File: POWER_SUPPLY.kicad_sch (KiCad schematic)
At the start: 4 parts, among them J1 Jack-DC, J2 USB_B_Micro, U4 LMR33640ADDA, U5 LMR33640ADDA

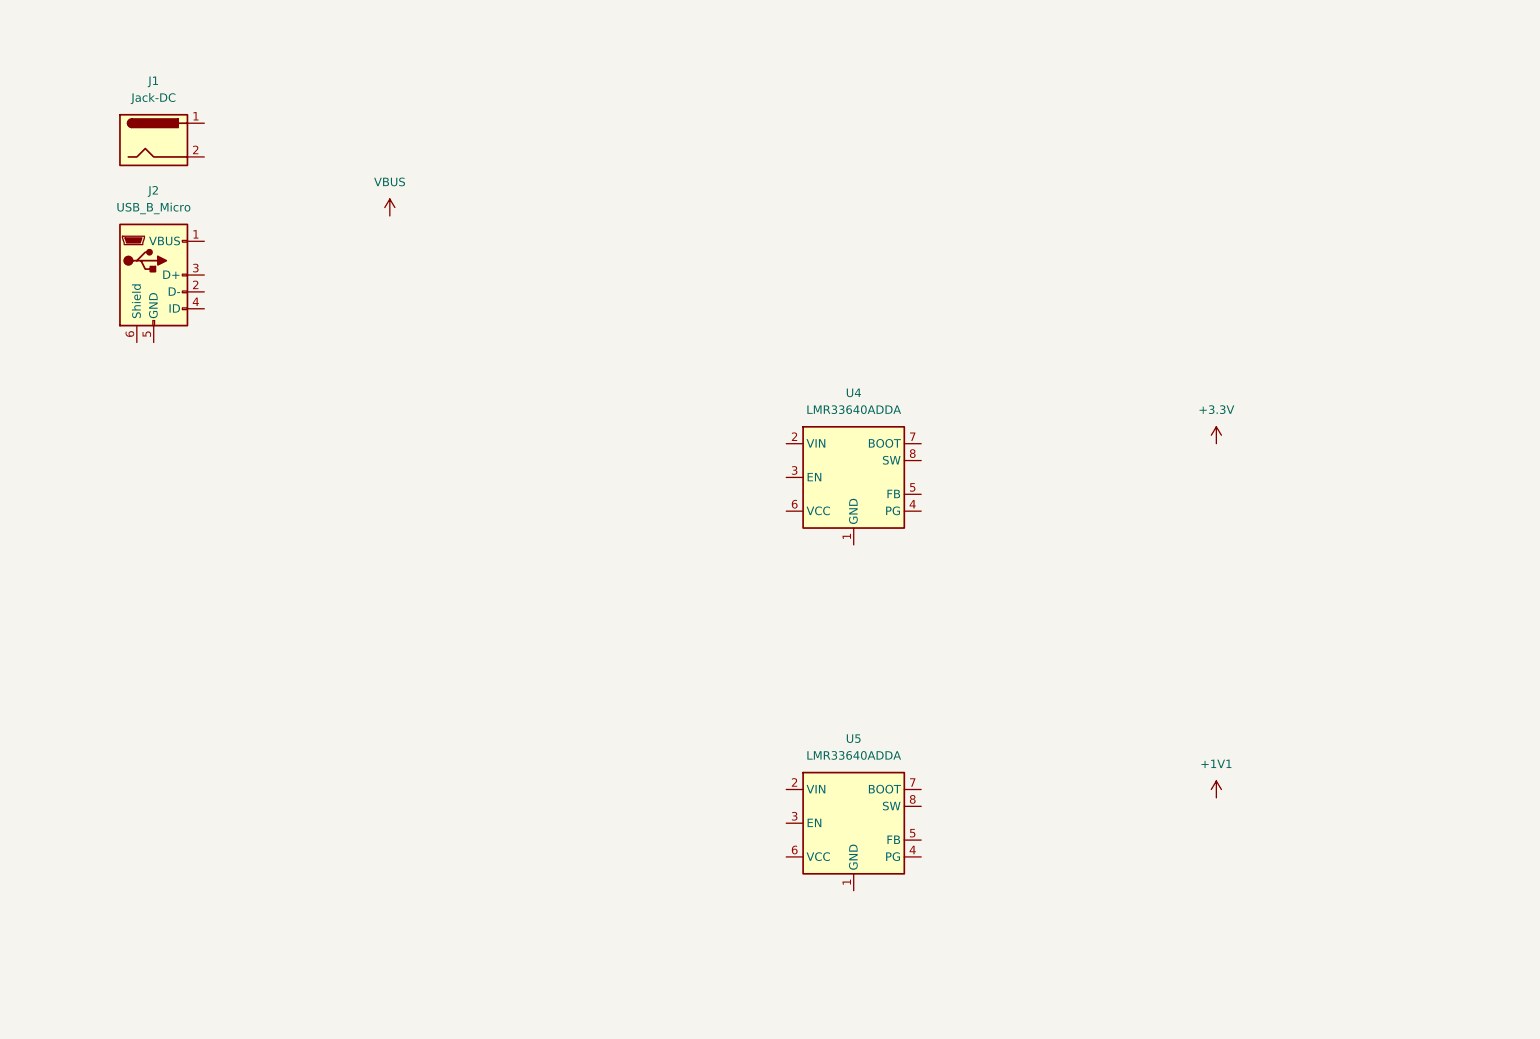
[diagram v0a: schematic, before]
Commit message: Weiter gearbeitet
Fast fertig:
HUB
Fertig
Connector (Up and Down)
MUX
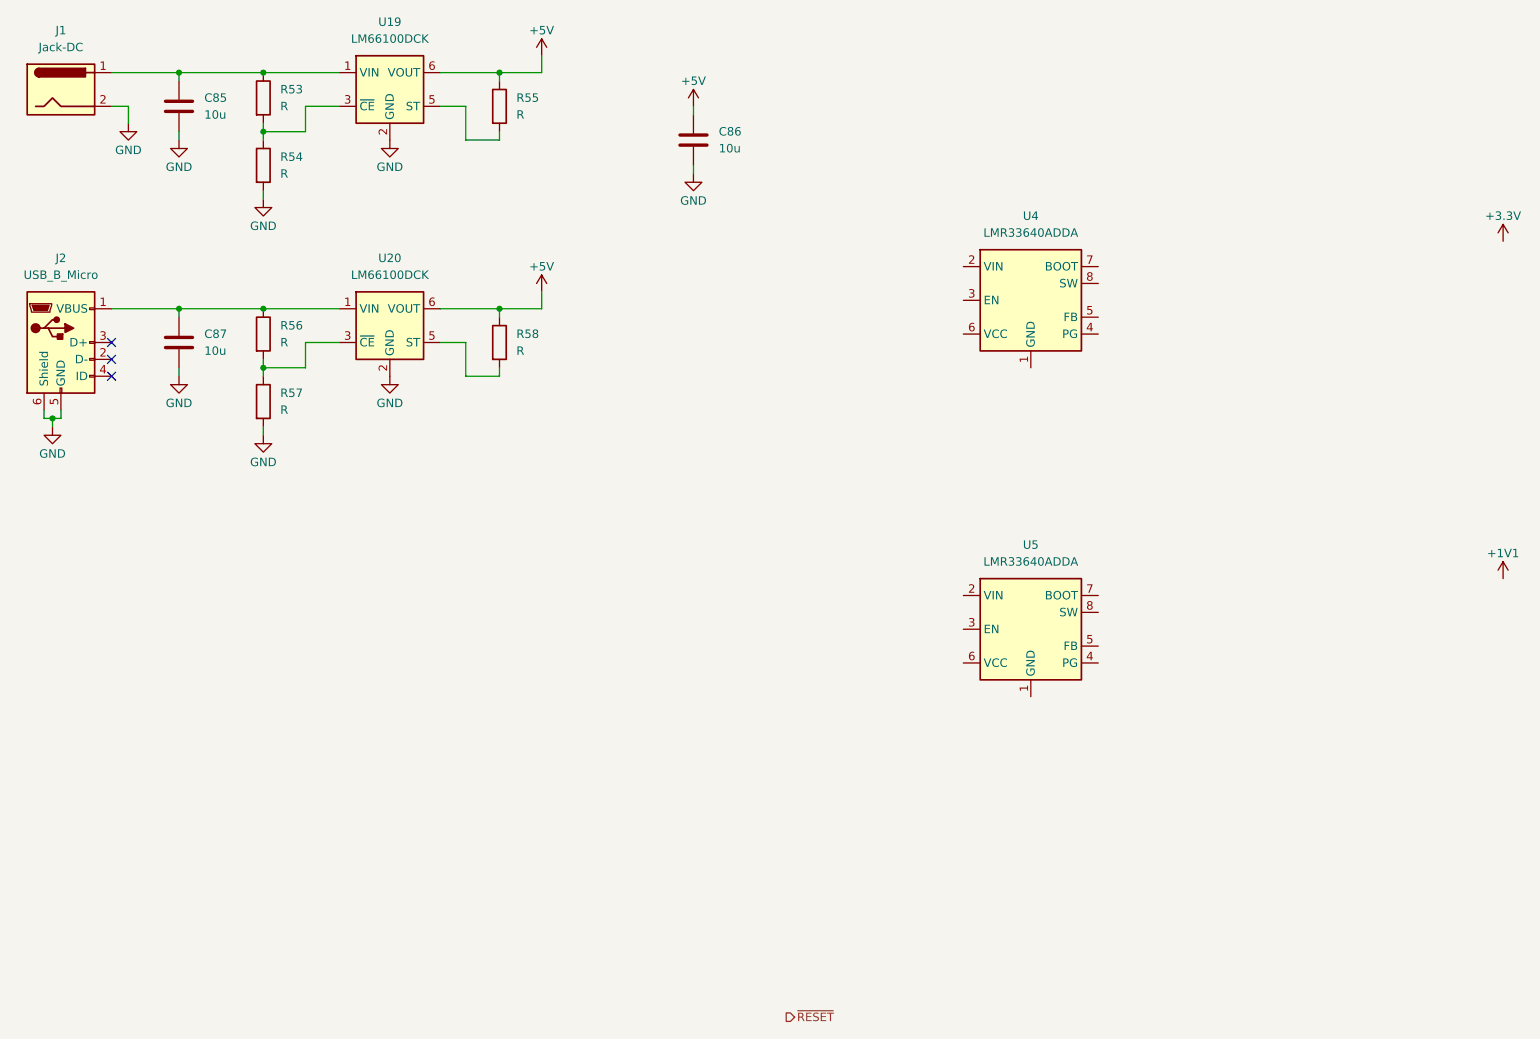
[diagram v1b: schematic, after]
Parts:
- added C85, C86, C87: 10u, Capacitor_SMD:C_0603_1608Metric, symbol Device:C
- added R53, R54, R55, R56, R57, R58: R, symbol Device:R
- added U19, U20: LM66100DCK, Package_TO_SOT_SMD:SOT-363_SC-70-6, symbol Power_Management:LM66100DCK
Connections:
- net at J2.1 (VBUS): now also C87.1, R56.1, U20.1 (VIN)
- net GND: now reaches J2.5 (GND)
- net GND: now also J1.2, J2.6 (Shield), C85.2, C86.2, C87.2, R54.2, R57.2, U19.2 (GND), U20.2 (GND)
- net at J1.1: now also C85.1, R53.1, U19.1 (VIN)
- new net: R55.2, U19.5 (ST)
- new net: R53.2, R54.1, U19.3 (~{CE})
- new net: R56.2, R57.1, U20.3 (~{CE})
- new net: R58.2, U20.5 (ST)
- new net +5V: C86.1, R55.1, R58.1, U19.6 (VOUT), U20.6 (VOUT)
- no-connect marks 0 -> 3
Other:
- moved on the sheet: J1, J2, U4, U5

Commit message: Footprints Updated
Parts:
- C85, C86, C87: footprint Capacitor_SMD:C_0603_1608Metric -> 00_Capacitor:Cap_0603
- R53, R54, R55, R56, R57, R58: footprint (none) -> 00_Resistor:Res_0402
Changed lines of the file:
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@@
 			)
 		)
-		(property "Footprint" ""
+		(property "Footprint" "00_Resistor:Res_0402"
 			(at 98.552 30.48 90)
 			(effects
@@
 			)
 		)
-		(property "Footprint" ""
+		(property "Footprint" "00_Resistor:Res_0402"
 			(at 62.992 39.37 90)
 			(effects
@@
 			)
 		)
-		(property "Footprint" "Capacitor_SMD:C_0603_1608Metric"
+		(property "Footprint" "00_Capacitor:Cap_0603"
 			(at 130.5052 39.37 0)
 			(effects
@@
 			)
 		)
-		(property "Footprint" "Capacitor_SMD:C_0603_1608Metric"
+		(property "Footprint" "00_Capacitor:Cap_0603"
 			(at 53.0352 34.29 0)
 			(effects
@@
 			)
 		)
-		(property "Footprint" ""
+		(property "Footprint" "00_Resistor:Res_0402"
 			(at 62.992 64.77 90)
 			(effects
@@
 			)
 		)
-		(property "Footprint" ""
+		(property "Footprint" "00_Resistor:Res_0402"
 			(at 62.992 29.21 90)
 			(effects
@@
 			)
 		)
-		(property "Footprint" "Capacitor_SMD:C_0603_1608Metric"
+		(property "Footprint" "00_Capacitor:Cap_0603"
 			(at 53.0352 69.85 0)
 			(effects
@@
 			)
 		)
-		(property "Footprint" ""
+		(property "Footprint" "00_Resistor:Res_0402"
 			(at 98.552 66.04 90)
 			(effects
@@
 			)
 		)
-		(property "Footprint" ""
+		(property "Footprint" "00_Resistor:Res_0402"
 			(at 62.992 74.93 90)
 			(effects
